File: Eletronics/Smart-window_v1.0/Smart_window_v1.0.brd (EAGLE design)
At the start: 12 x 30 mm, 32 parts, among them IC1 SI7021-, SW1 PUSHBUTTON_3X3_SMALL_FOOTPRINT, SW2 PUSHBUTTON_3X3_SMALL_FOOTPRINT, U1 AP7340-18FS4-7

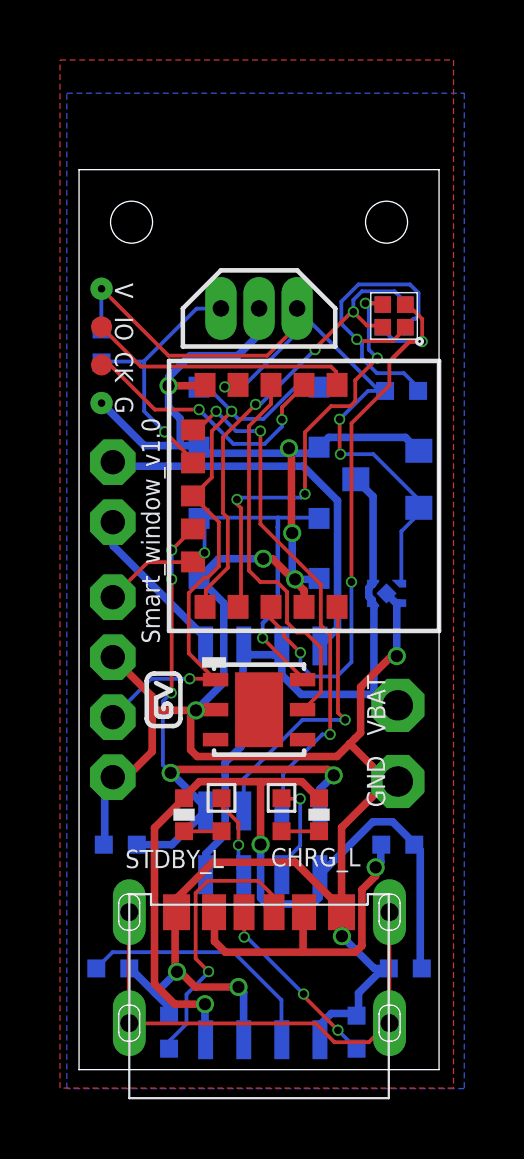
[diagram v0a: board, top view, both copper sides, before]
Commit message: Smart_window_v1.0
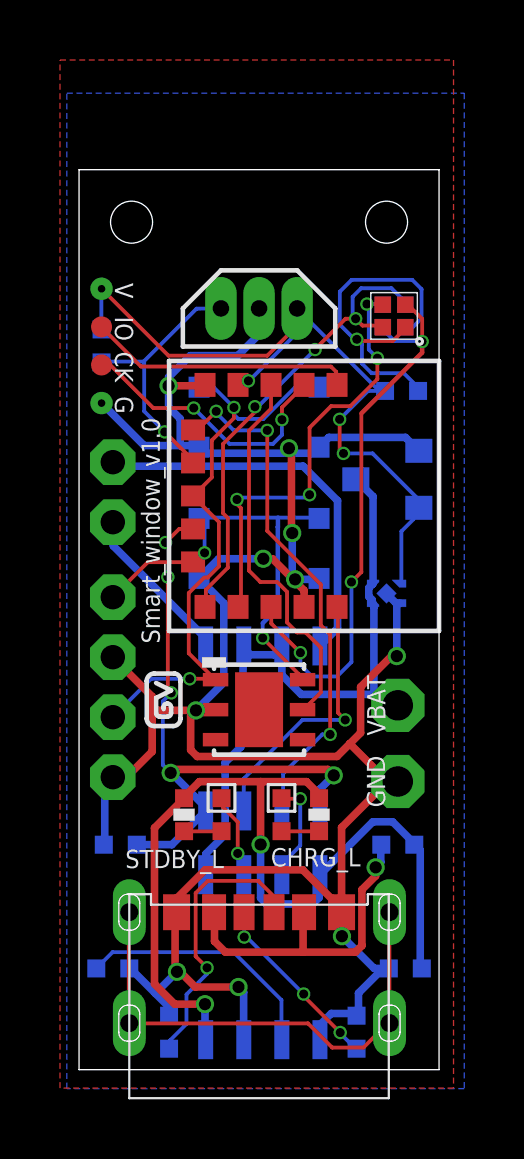
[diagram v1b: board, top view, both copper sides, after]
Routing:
- net 3V3: track 27.7 -> 26.7 mm
- net N$1: track 10.7 -> 11.6 mm
